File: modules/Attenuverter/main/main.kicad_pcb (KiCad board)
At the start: 2 copper layers, 40.3 x 111.8 mm, 40 parts, among them J1 IN, J2 Power, J3 OUT, Q1 BC547, Q2 BC547, Q3 BC547, Q4 BC547, U1 LM358, U2 ICM7555

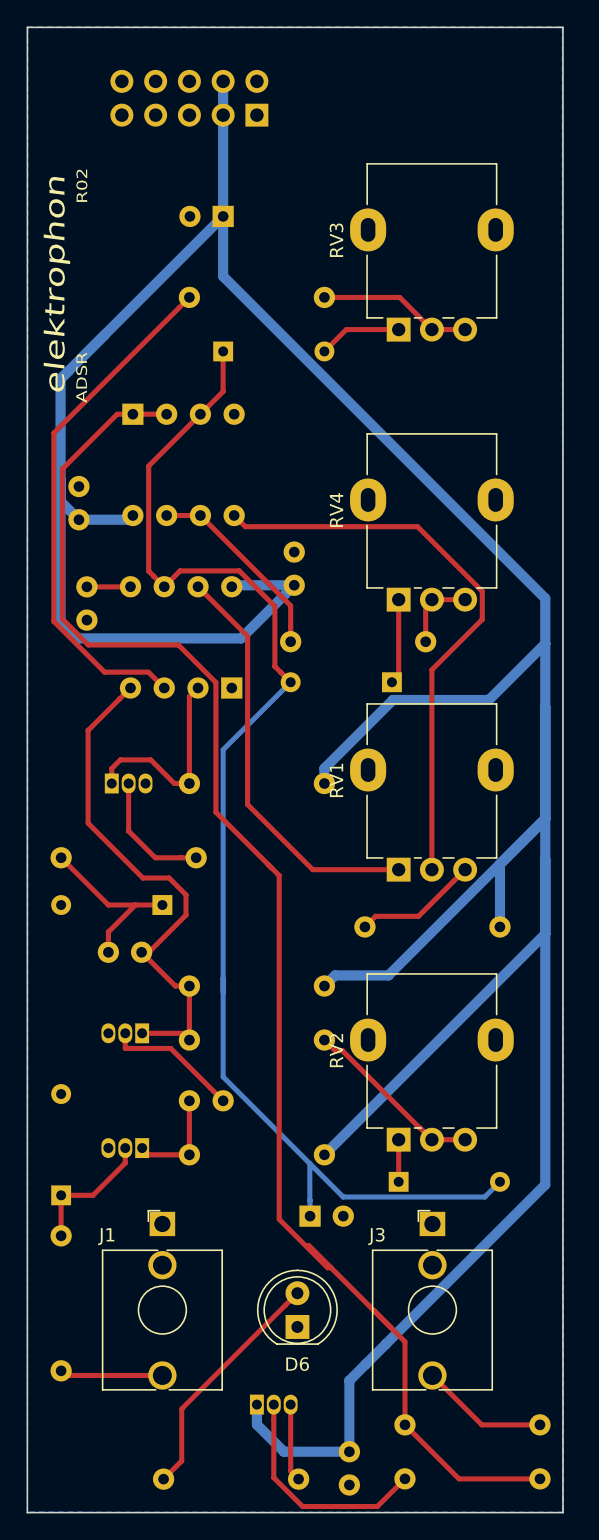
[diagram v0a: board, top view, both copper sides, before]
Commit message: update schema
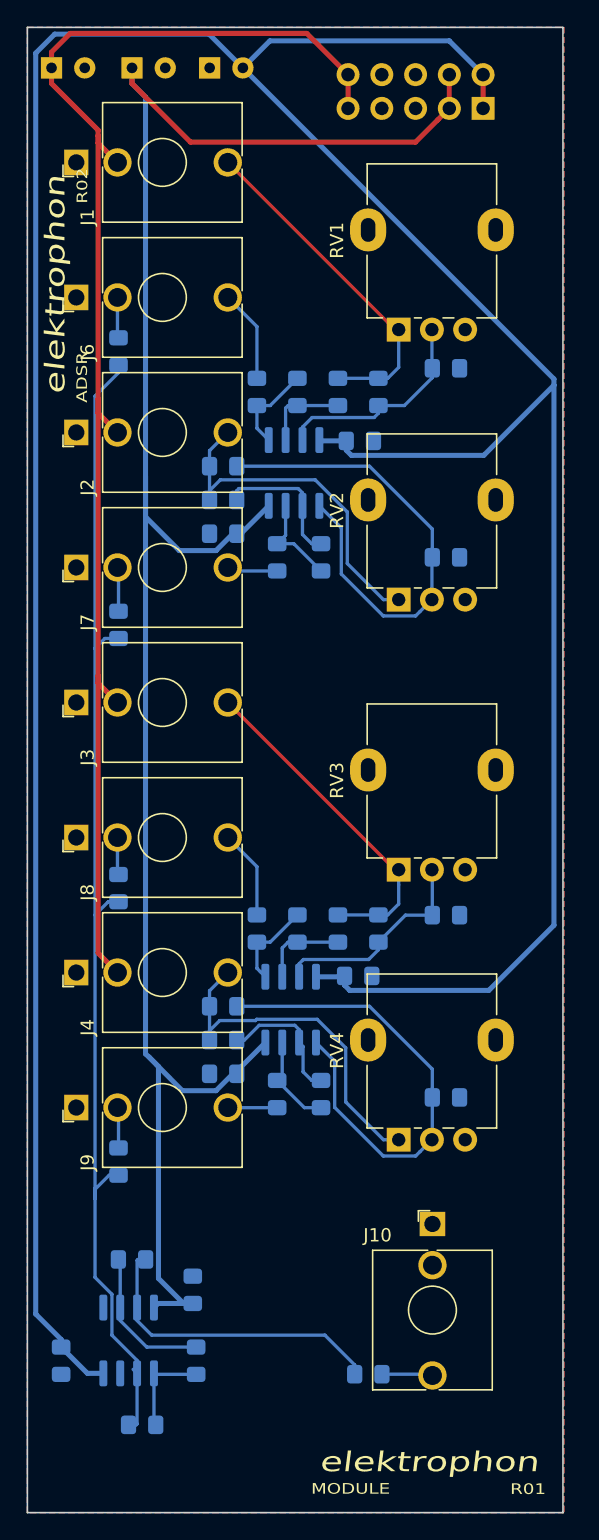
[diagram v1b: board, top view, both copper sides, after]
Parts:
- removed D1, D2, D3, D4, D5: D, Diode_THT:D_DO-34_SOD68_P7.62mm_Horizontal
- removed D6: LED, LED_THT:LED_D5.0mm
- removed Q1, Q2, Q3, Q4: BC547, Package_TO_SOT_THT:TO-92_Inline
- added C8: 0.1u, Capacitor_SMD:C_0805_2012Metric_Pad1.15x1.40mm_HandSolder, B.Cu at (53.3, 151.1)
- added C9: 10u, Capacitor_THT:CP_Radial_D5.0mm_P2.50mm, B.Cu at (52.6, 53.8)
- added J10: OUT, elektrophon:Jack_3.5mm_WQP-PJ398SM_Vertical, F.Cu at (81.3, 147.3)
- added J3: IN, elektrophon:Jack_3.5mm_WQP-PJ398SM_Vertical, F.Cu at (61.0, 101.6)
- added J4: IN, elektrophon:Jack_3.5mm_WQP-PJ398SM_Vertical, F.Cu at (61.0, 121.9)
- added J5: IDC Header, Connector_IDC:IDC-Header_2x05_P2.54mm_Vertical, B.Cu at (85.1, 56.9)
- added J7: OUT, elektrophon:Jack_3.5mm_WQP-PJ398SM_Vertical, F.Cu at (61.0, 91.4)
- added J8: OUT, elektrophon:Jack_3.5mm_WQP-PJ398SM_Vertical, F.Cu at (61.0, 111.8)
- added J9: OUT, elektrophon:Jack_3.5mm_WQP-PJ398SM_Vertical, F.Cu at (61.0, 132.1)
- added R13: 100k, Resistor_SMD:R_0805_2012Metric_Pad1.15x1.40mm_HandSolder, B.Cu at (71.1, 78.2)
- added R14: 100k, Resistor_SMD:R_0805_2012Metric_Pad1.15x1.40mm_HandSolder, B.Cu at (72.9, 90.7)
- added R15: 100k, Resistor_SMD:R_0805_2012Metric_Pad1.15x1.40mm_HandSolder, B.Cu at (71.1, 118.6)
- added R16: 100k, Resistor_SMD:R_0805_2012Metric_Pad1.15x1.40mm_HandSolder, B.Cu at (72.9, 131.1)
- added R18: 1k, Resistor_SMD:R_0805_2012Metric_Pad1.15x1.40mm_HandSolder, B.Cu at (69.6, 90.7)
- added R19: 1k, Resistor_SMD:R_0805_2012Metric_Pad1.15x1.40mm_HandSolder, B.Cu at (68.1, 118.6)
- added R20: 1k, Resistor_SMD:R_0805_2012Metric_Pad1.15x1.40mm_HandSolder, B.Cu at (69.6, 131.1)
- added R21: 100k, Resistor_SMD:R_0805_2012Metric_Pad1.15x1.40mm_HandSolder, B.Cu at (57.7, 75.2)
- added R22: 100k, Resistor_SMD:R_0805_2012Metric_Pad1.15x1.40mm_HandSolder, B.Cu at (57.7, 95.8)
- added R23: 100k, Resistor_SMD:R_0805_2012Metric_Pad1.15x1.40mm_HandSolder, B.Cu at (57.7, 115.6)
- added R24: 100k, Resistor_SMD:R_0805_2012Metric_Pad1.15x1.40mm_HandSolder, B.Cu at (57.7, 136.1)
- added R25: 100k, Resistor_SMD:R_0805_2012Metric_Pad1.15x1.40mm_HandSolder, B.Cu at (59.4, 156.0)
- added R26: 100k, Resistor_SMD:R_0805_2012Metric_Pad1.15x1.40mm_HandSolder, B.Cu at (63.5, 151.1)
- added R27: 100k, Resistor_SMD:R_0805_2012Metric_Pad1.15x1.40mm_HandSolder, B.Cu at (58.7, 143.5)
- added R28: 1k, Resistor_SMD:R_0805_2012Metric_Pad1.15x1.40mm_HandSolder, B.Cu at (76.5, 152.1)
- added REF**: elektrophon logo, elektrophon:elektrophon logo, F.Cu at (81.0, 159.8)
- added U3: OPA2134, Package_SO:SOIC-8_3.9x4.9mm_P1.27mm, B.Cu at (58.4, 149.6)
- C2: value 0.1u -> 10u; footprint Capacitor_THT:C_Disc_D3.4mm_W2.1mm_P2.50mm -> Capacitor_THT:CP_Radial_D5.0mm_P2.50mm
- C3: footprint Capacitor_THT:C_Disc_D3.4mm_W2.1mm_P2.50mm -> Capacitor_SMD:C_0805_2012Metric_Pad1.15x1.40mm_HandSolder
- C4, C5: value 10n -> 0.1u; footprint Capacitor_THT:C_Disc_D3.4mm_W2.1mm_P2.50mm -> Capacitor_SMD:C_0805_2012Metric_Pad1.15x1.40mm_HandSolder
- C6: value 4u7 -> 0.1u; footprint Capacitor_THT:CP_Radial_D5.0mm_P2.50mm -> Capacitor_SMD:C_0805_2012Metric_Pad1.15x1.40mm_HandSolder
- C7: value 100n -> 0.1u; footprint Capacitor_THT:C_Disc_D3.4mm_W2.1mm_P2.50mm -> Capacitor_SMD:C_0805_2012Metric_Pad1.15x1.40mm_HandSolder
- J1: footprint elektrophon:Jack_3.5mm_QingPu_WQP-PJ398SM_Vertical_CircularHoles -> elektrophon:Jack_3.5mm_WQP-PJ398SM_Vertical
- J2: value Power -> IN; footprint Connector_IDC:IDC-Header_2x05_P2.54mm_Vertical -> elektrophon:Jack_3.5mm_WQP-PJ398SM_Vertical; moved to F.Cu
- J6: renamed from J3; footprint elektrophon:Jack_3.5mm_QingPu_WQP-PJ398SM_Vertical_CircularHoles -> elektrophon:Jack_3.5mm_WQP-PJ398SM_Vertical
- R1, R5: value 10k -> 47k; footprint Resistor_THT:R_Axial_DIN0207_L6.3mm_D2.5mm_P10.16mm_Horizontal -> Resistor_SMD:R_0805_2012Metric_Pad1.15x1.40mm_HandSolder
- R10: value 100 -> 100k; footprint Resistor_THT:R_Axial_DIN0207_L6.3mm_D2.5mm_P10.16mm_Horizontal -> Resistor_SMD:R_0805_2012Metric_Pad1.15x1.40mm_HandSolder
- R11: value 10k -> 100k; footprint Resistor_THT:R_Axial_DIN0207_L6.3mm_D2.5mm_P10.16mm_Horizontal -> Resistor_SMD:R_0805_2012Metric_Pad1.15x1.40mm_HandSolder
- R12: value 2k2 -> 100k; footprint Resistor_THT:R_Axial_DIN0207_L6.3mm_D2.5mm_P10.16mm_Horizontal -> Resistor_SMD:R_0805_2012Metric_Pad1.15x1.40mm_HandSolder
- R17: renamed from R13; footprint Resistor_THT:R_Axial_DIN0207_L6.3mm_D2.5mm_P10.16mm_Horizontal -> Resistor_SMD:R_0805_2012Metric_Pad1.15x1.40mm_HandSolder
- R2, R4, R6: value 4k7 -> 47k; footprint Resistor_THT:R_Axial_DIN0207_L6.3mm_D2.5mm_P10.16mm_Horizontal -> Resistor_SMD:R_0805_2012Metric_Pad1.15x1.40mm_HandSolder
- R3: value 22k -> 47k; footprint Resistor_THT:R_Axial_DIN0207_L6.3mm_D2.5mm_P2.54mm_Vertical -> Resistor_SMD:R_0805_2012Metric_Pad1.15x1.40mm_HandSolder
- R7, R8: value 100 -> 47k; footprint Resistor_THT:R_Axial_DIN0207_L6.3mm_D2.5mm_P10.16mm_Horizontal -> Resistor_SMD:R_0805_2012Metric_Pad1.15x1.40mm_HandSolder
- R9: value 4k7 -> 100k; footprint Resistor_THT:R_Axial_DIN0207_L6.3mm_D2.5mm_P10.16mm_Horizontal -> Resistor_SMD:R_0805_2012Metric_Pad1.15x1.40mm_HandSolder
- RV1: value 10k -> 100k
- RV2, RV3, RV4: value 1M LOG -> 100k
- U1: value LM358 -> OPA2134; footprint Package_DIP:DIP-8_W7.62mm_Socket -> Package_SO:SOIC-8_3.9x4.9mm_P1.27mm
- U2: value ICM7555 -> OPA2134; footprint Package_DIP:DIP-8_W7.62mm_Socket -> Package_SO:SOIC-8_3.9x4.9mm_P1.27mm
- moved J1 86.4 mm to (61.0, 61.0), turned to 90 degrees
- moved J6 78.9 mm to (61.0, 71.1), turned to 90 degrees
- moved R17 78.5 mm to (68.1, 78.2), turned to 90 degrees
- moved R1 67.8 mm to (77.2, 78.2)
- moved R8 60.9 mm to (82.3, 131.3), turned to 0 degrees
- moved R2 59.9 mm to (82.3, 76.5), turned to 0 degrees
- moved R3 47.8 mm to (65.5, 83.8), turned to 0 degrees
- moved C4 42.9 mm to (75.8, 81.9), turned to 180 degrees
- moved R11 41.7 mm to (74.2, 118.6), turned to 90 degrees
- moved RV1 40.6 mm to (81.3, 66.0)
- moved RV2 40.6 mm to (81.3, 86.4)
- moved RV3 40.6 mm to (81.3, 106.7)
- moved RV4 40.6 mm to (81.3, 127.0)
- moved R9 40.3 mm to (74.2, 78.2), turned to 90 degrees
- moved C5 35.6 mm to (65.5, 129.5), turned to 180 degrees
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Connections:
- C2 pad 2: +15V -> -15V
- C4 pad 1: Net-(C4-Pad1) -> GND
- C4 pad 2: Net-(C4-Pad2) -> -15V
- C5 pad 1: GND -> +15V
- C5 pad 2: Net-(C5-Pad2) -> GND
- C6 pad 1: Net-(C6-Pad1) -> GND
- C6 pad 2: GND -> -15V
- J1 pad TN: Net-(J1-PadTN) -> +5V
- J6 pad TN: Net-(J3-PadTN) -> /MIX_1
- R1 pad 1: Net-(D1-Pad1) -> Net-(J1-PadT)
- R1 pad 2: Net-(J1-PadT) -> Net-(R1-Pad2)
- R10 pad 2: Net-(R10-Pad2) -> Net-(J2-PadT)
- R11 pad 1: Net-(Q4-Pad2) -> Net-(R11-Pad1)
- R11 pad 2: Net-(R11-Pad2) -> Net-(J3-PadT)
- R12 pad 1: Net-(Q4-Pad3) -> Net-(R12-Pad1)
- R12 pad 2: Net-(D6-Pad2) -> Net-(J4-PadT)
- R17 pad 1: Net-(R11-Pad2) -> Net-(R13-Pad1)
- R2 pad 1: +15V -> Net-(R1-Pad2)
- R2 pad 2: Net-(Q1-Pad1) -> GND
- R3 pad 1: Net-(Q2-Pad2) -> Net-(J2-PadT)
- R3 pad 2: Net-(Q1-Pad1) -> Net-(R3-Pad2)
- R4 pad 1: +15V -> Net-(R3-Pad2)
- R4 pad 2: Net-(C4-Pad2) -> GND
- R5 pad 1: Net-(Q3-Pad2) -> Net-(J3-PadT)
- R5 pad 2: Net-(C4-Pad1) -> Net-(R5-Pad2)
- R6 pad 1: +15V -> Net-(R5-Pad2)
- R6 pad 2: Net-(Q3-Pad1) -> GND
- R7 pad 1: Net-(R7-Pad1) -> Net-(J4-PadT)
- R7 pad 2: Net-(C4-Pad2) -> Net-(R7-Pad2)
- R8 pad 1: Net-(R8-Pad1) -> Net-(R7-Pad2)
- R8 pad 2: Net-(R8-Pad2) -> GND
- R9 pad 1: Net-(R9-Pad1) -> Net-(R13-Pad2)
- R9 pad 2: +15V -> Net-(J1-PadT)
- RV1 pad 1: Net-(RV1-Pad1) -> Net-(J1-PadT)
- RV1 pad 2: Net-(RV1-Pad2) -> Net-(R1-Pad2)
- RV1 pad 3: Net-(R9-Pad1) -> GND
- RV2 pad 1: Net-(D3-Pad1) -> Net-(J2-PadT)
- RV2 pad 2: Net-(R7-Pad1) -> Net-(R3-Pad2)
- RV2 pad 3: Net-(R7-Pad1) -> GND
- RV3 pad 1: Net-(D4-Pad2) -> Net-(J3-PadT)
- RV3 pad 2: Net-(R8-Pad1) -> Net-(R5-Pad2)
- RV3 pad 3: Net-(R8-Pad1) -> GND
- RV4 pad 1: Net-(D5-Pad1) -> Net-(J4-PadT)
- RV4 pad 2: Net-(R10-Pad2) -> Net-(R7-Pad2)
- RV4 pad 3: Net-(R10-Pad2) -> GND
- U1 pad 1: Net-(R11-Pad2) -> Net-(R13-Pad1)
- U1 pad 2: Net-(R11-Pad2) -> Net-(R13-Pad2)
- U1 pad 3: Net-(C6-Pad1) -> Net-(R1-Pad2)
- U1 pad 4: GND -> -15V
- U1 pad 5: Net-(RV1-Pad2) -> Net-(R3-Pad2)
- U1 pad 7: Net-(R10-Pad1) -> Net-(R14-Pad1)
- U2 pad 1: GND -> Net-(R15-Pad1)
- U2 pad 2: Net-(Q3-Pad1) -> Net-(R11-Pad1)
- U2 pad 3: Net-(R8-Pad2) -> Net-(R5-Pad2)
- U2 pad 4: Net-(C4-Pad2) -> -15V
- U2 pad 5: Net-(C5-Pad2) -> Net-(R7-Pad2)
- U2 pad 6: Net-(C6-Pad1) -> Net-(R12-Pad1)
- U2 pad 7: Net-(RV1-Pad1) -> Net-(R16-Pad1)
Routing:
- net -15V: track 0.00 -> 257.7 mm
- net +15V: track 290.0 -> 155.0 mm
- net Net-(R11-Pad2): track 112.8 -> 0.00 mm
- net +5V: track 0.00 -> 106.4 mm
- net Net-(C6-Pad1): track 98.5 -> 0.00 mm
- net Net-(R21-Pad2): track 0.00 -> 90.7 mm
- net Net-(RV1-Pad2): track 43.5 -> 0.00 mm
- net Net-(C4-Pad2): track 39.6 -> 0.00 mm
- net Net-(R8-Pad2): track 39.0 -> 0.00 mm
- net Net-(R7-Pad2): track 0.00 -> 36.8 mm
- net Net-(R3-Pad2): track 0.00 -> 36.4 mm
- net Net-(RV1-Pad1): track 31.3 -> 0.00 mm
- net Net-(J4-PadT): track 0.00 -> 27.1 mm
- net Net-(J2-PadT): track 0.00 -> 26.9 mm
- net Net-(J3-PadT): track 0.00 -> 25.6 mm
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- added copper zone on F.Cu, net GND
